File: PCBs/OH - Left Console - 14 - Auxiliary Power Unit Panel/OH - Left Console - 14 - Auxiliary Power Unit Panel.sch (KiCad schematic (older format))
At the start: 10 parts, among them J1 Input Columns, J2 Input Rows, SW1 EXT_PWR_SW

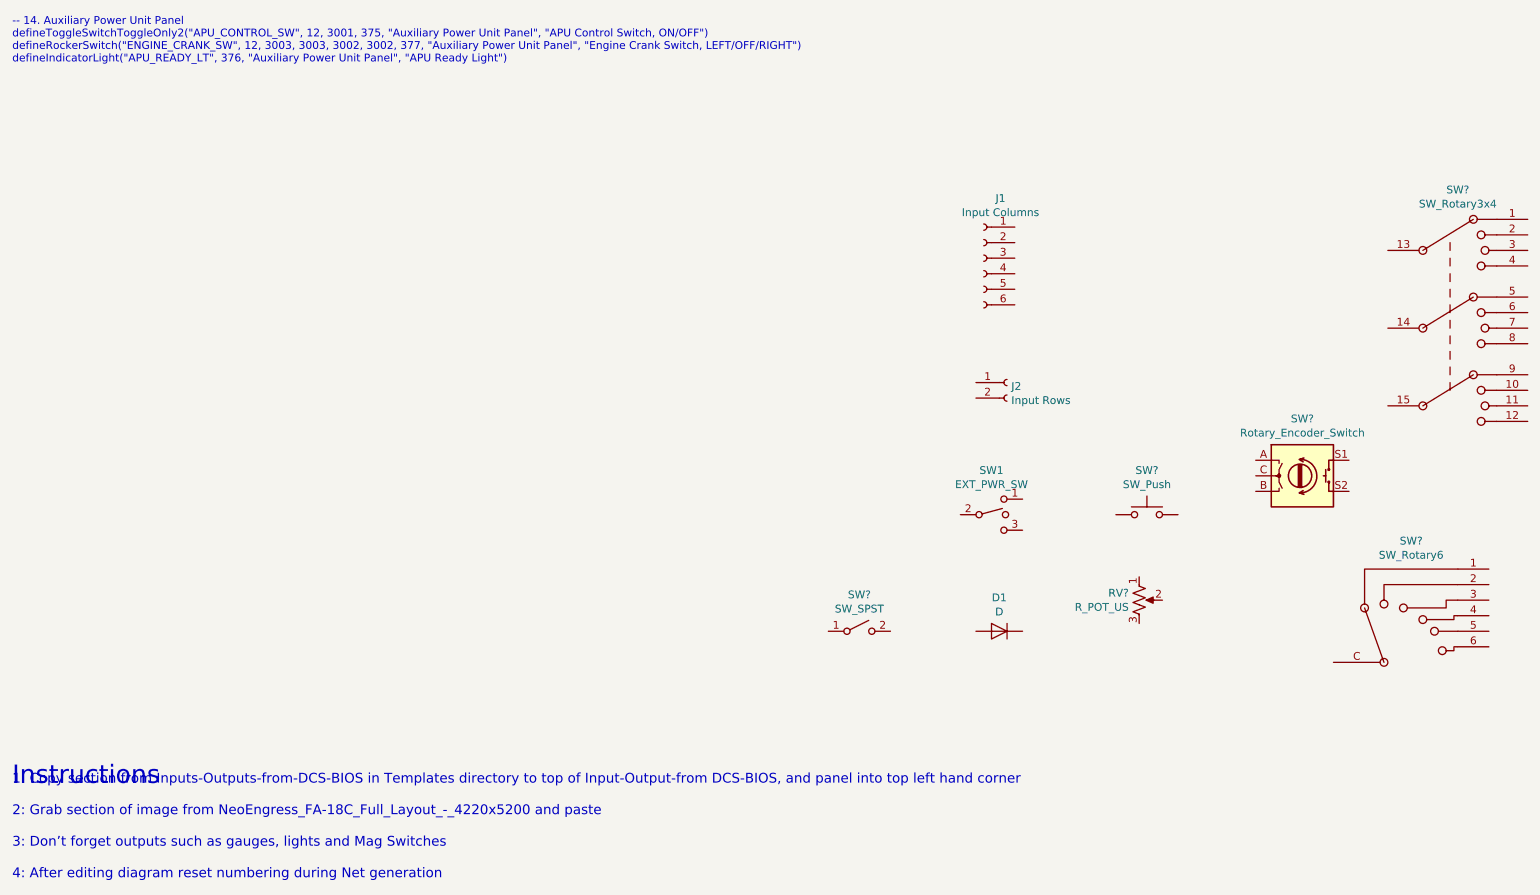
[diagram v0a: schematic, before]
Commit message: Panels
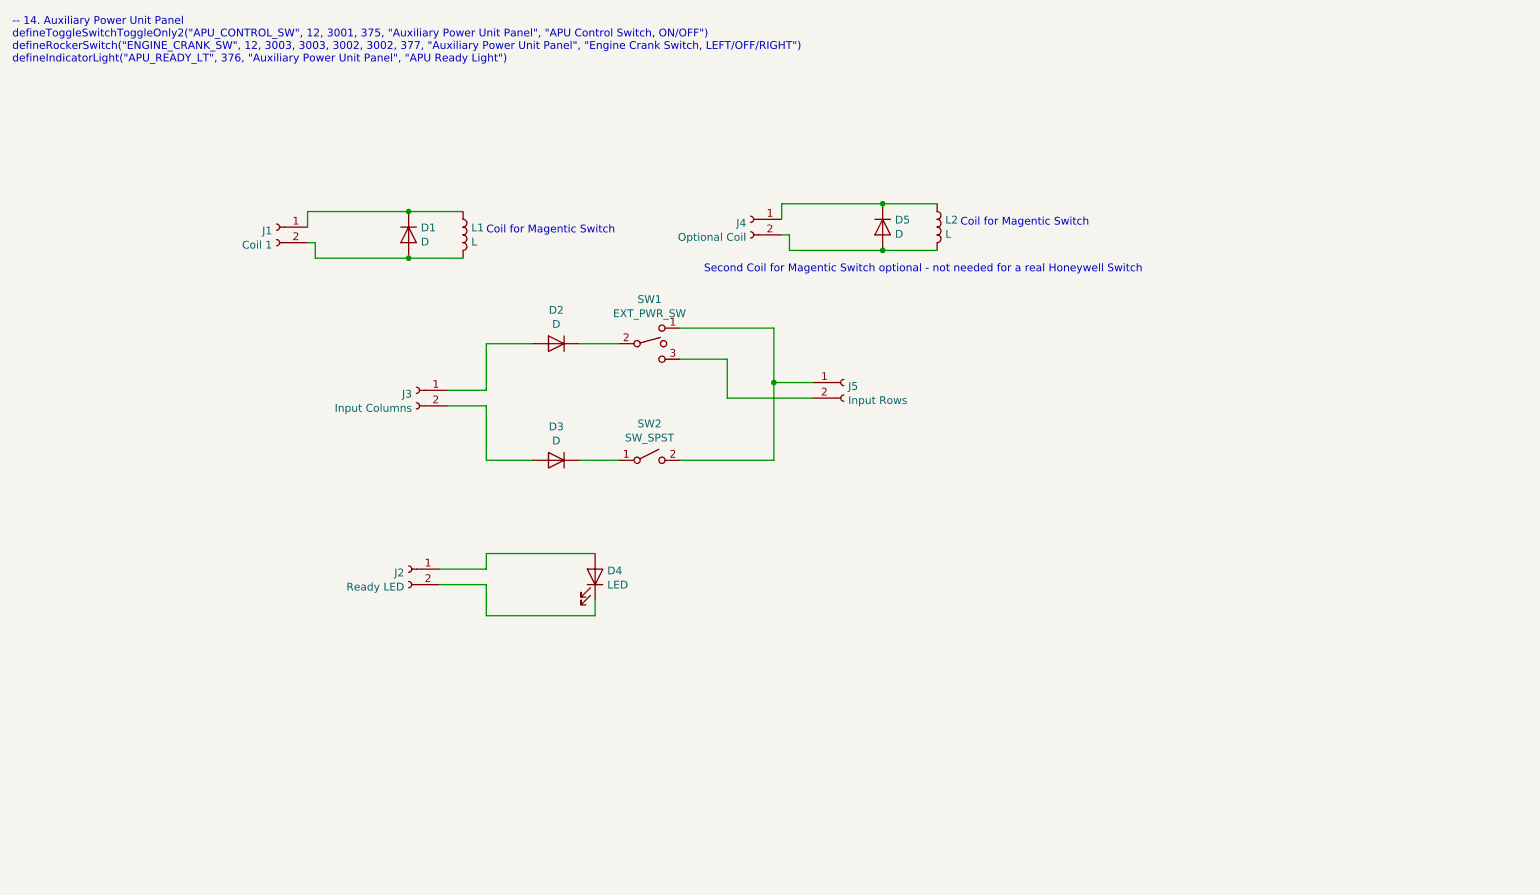
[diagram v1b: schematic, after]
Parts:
- removed J1: Input Columns, PT_Library_v001:Molex_1x06_P2.54mm_Vertical, symbol Connector:Conn_01x06_Female
- removed RV?: R_POT_US, PT_Library_v001:Molex_1x03_P2.54mm_Vertical, symbol Device:R_POT_US
- removed SW?: SW_Push, PT_Library_v001:Molex_1x02_P2.54mm_Vertical, symbol Switch:SW_Push
- removed SW?: Rotary_Encoder_Switch, PT_Library_v001:Molex_1x03_P2.54mm_Vertical, symbol Device:Rotary_Encoder_Switch
- removed SW?: SW_Rotary6, symbol OpenHornet2:SW_Rotary6
- removed SW?: SW_Rotary3x4, symbol Switch:SW_Rotary3x4
- added D1, D5: D, Diode_THT:D_DO-41_SOD81_P10.16mm_Horizontal, symbol Diode:1N4001
- added D3: D, PT_Library_v001:D_Signal_P7.62mm_Horizontal, symbol Device:D
- added D4: LED, symbol Device:LED
- added J1: Coil 1, PT_Library_v001:Molex_1x02_P2.54mm_Vertical, symbol Connector:Conn_01x02_Female
- added J2: Ready LED, PT_Library_v001:Molex_1x02_P2.54mm_Vertical, symbol Connector:Conn_01x02_Female
- added J3: Input Columns, PT_Library_v001:Molex_1x02_P2.54mm_Vertical, symbol Connector:Conn_01x02_Female
- added J4: Optional Coil, PT_Library_v001:Molex_1x02_P2.54mm_Vertical, symbol Connector:Conn_01x02_Female
- added L1, L2: L, symbol Device:L
- gave numbers to parts that had none: 1
- renumbered D1 to D2, J2 to J5
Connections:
- net at SW1.1: now also J5.1 (Pin_1), SW2.2 (B)
- net at SW1.2: now also D2.1 (K)
- net at SW1.3: now also J5.2 (Pin_2)
- net at D2.2 (A): now also J3.1 (Pin_1)
- net at SW2.1 (A): now also D3.1 (K)
- new net: D3.2 (A), J3.2 (Pin_2)
- new net: D4.1 (K), J2.2 (Pin_2)
- new net: D4.2 (A), J2.1 (Pin_1)
- new net: D5.1 (K), J4.1 (Pin_1), L2.1
- new net: D5.2 (A), J4.2 (Pin_2), L2.2
- new net: D1.1 (K), J1.1 (Pin_1), L1.1
- new net: D1.2 (A), J1.2 (Pin_2), L1.2
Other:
- note added: "Coil for Magentic Switch"
- note added: "Second Coil for Magentic Switch optional - not needed for a real Honeywell Switch"
- note removed: "1: Copy section from Inputs-Outputs-from-DCS-BIOS in Templates directory to top of Input-Output-from DCS-BIOS, and panel into top left hand corner\n\n2: Grab section of image from NeoEngress_FA-18C_Full_Layout_-_4220x5200 and paste \n\n3: Don’t forget outputs such as gauges, lights and Mag Switches\n\n4: After editing diagram reset numbering during Net generation\n"
- note removed: "Instructions"
- moved on the sheet: D2, J5, SW1, SW2
